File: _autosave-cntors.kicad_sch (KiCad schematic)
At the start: 3 parts, among them J2 LP-XDS110_Debug_Conn, J3 UART_debug

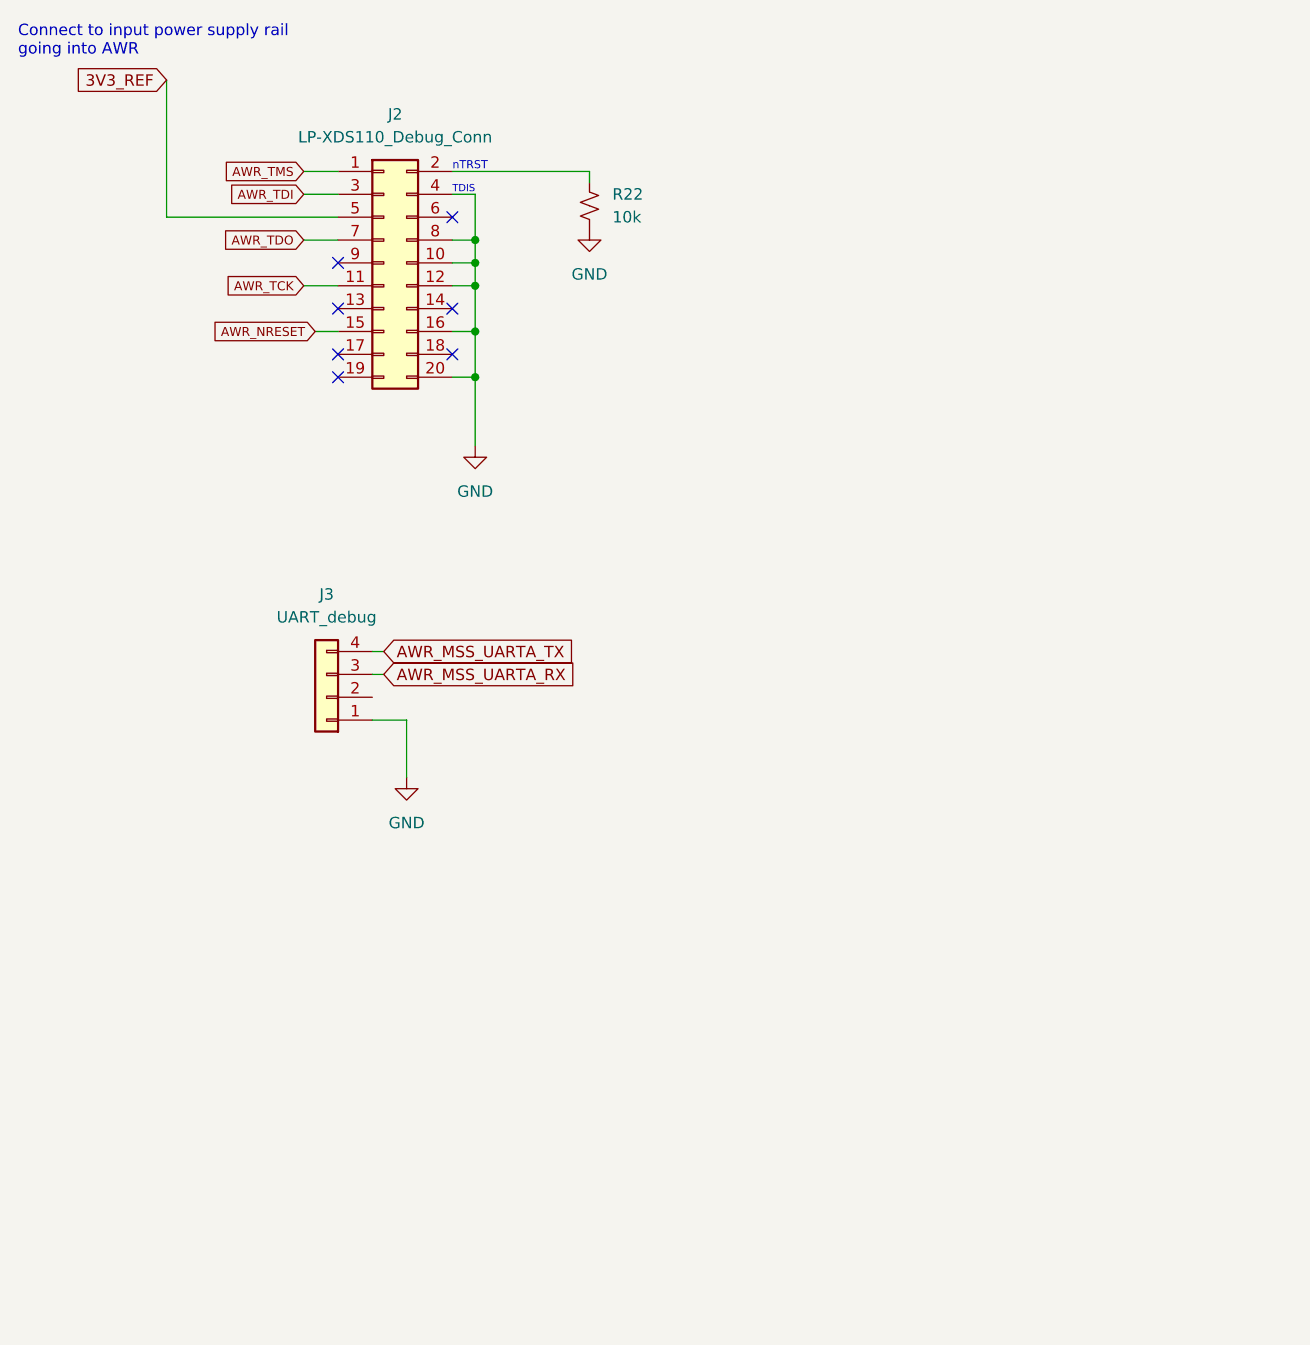
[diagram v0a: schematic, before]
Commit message: finishing connectors
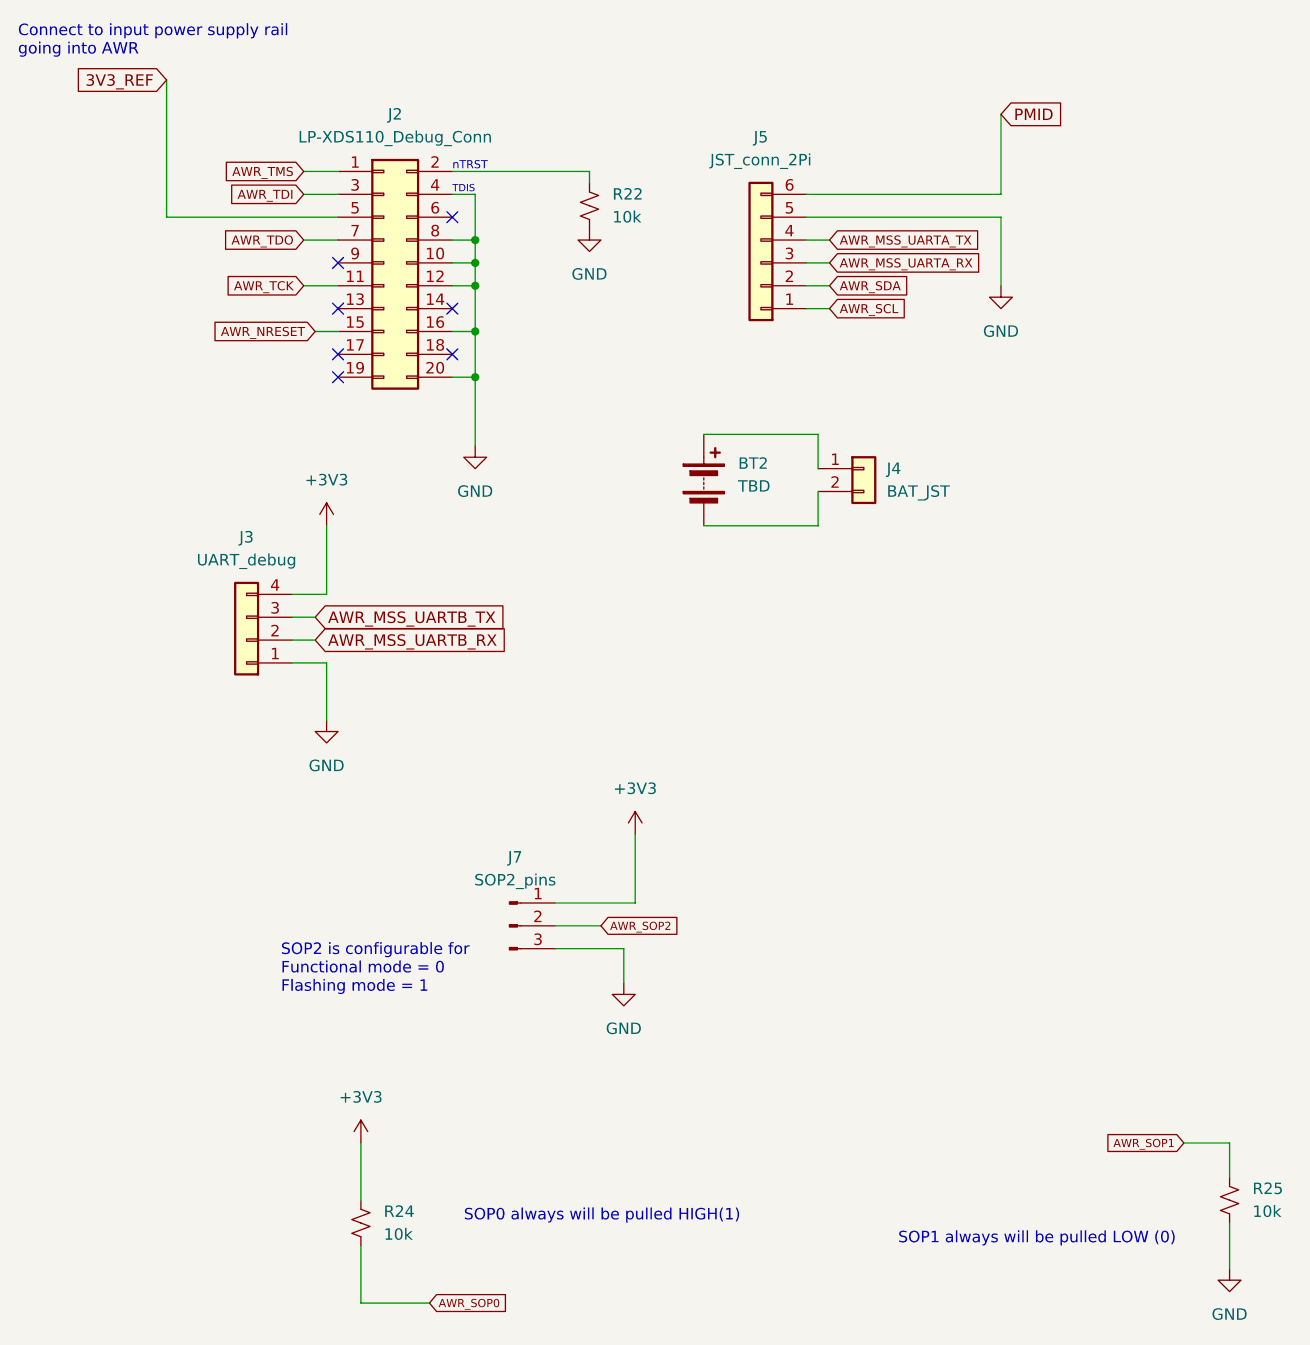
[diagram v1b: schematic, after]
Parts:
- added BT2: TBD, symbol Device:Battery
- added J4: BAT_JST, symbol Connector_Generic:Conn_01x02
- added J5: JST_conn_2Pi, symbol Connector_Generic:Conn_01x06
- added J7: SOP2_pins, symbol Connector:Conn_01x03_Pin
- added R24, R25: 10k, symbol Device:R_Small_US
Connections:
- net AWR_MSS_UARTA_RX: now also J5.3 (Pin_3); no longer J3.3 (Pin_3)
- net AWR_MSS_UARTA_TX: now also J5.4 (Pin_4); no longer J3.4 (Pin_4)
- net GND: now also J5.5 (Pin_5), J7.3 (Pin_3), R25.1
- net AWR_MSS_UARTB_RX: now reaches J3.2 (Pin_2)
- new net: BT2.1 (+), J4.1 (Pin_1)
- new net: BT2.2 (-), J4.2 (Pin_2)
- new net +3V3: J3.4 (Pin_4), J7.1 (Pin_1), R24.1
- new net AWR_MSS_UARTB_TX: J3.3 (Pin_3)
- new net AWR_SCL: J5.1 (Pin_1)
- new net AWR_SDA: J5.2 (Pin_2)
- new net AWR_SOP0: R24.2
- new net AWR_SOP1: R25.2
- new net AWR_SOP2: J7.2 (Pin_2)
- new net PMID: J5.6 (Pin_6)
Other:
- note added: "SOP0 always will be pulled HIGH(1)"
- note added: "SOP1 always will be pulled LOW (0)"
- note added: "SOP2 is configurable for Functional mode = 0 Flashing mode = 1"
- moved on the sheet: J3
